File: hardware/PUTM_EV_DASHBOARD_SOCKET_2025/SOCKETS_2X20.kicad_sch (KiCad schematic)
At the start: 10 parts, among them J1pin200000 Conn_02x20_Top_Bottom_Mountin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, J2SO2 Conn_02x20_Top_Bottom_Mountin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

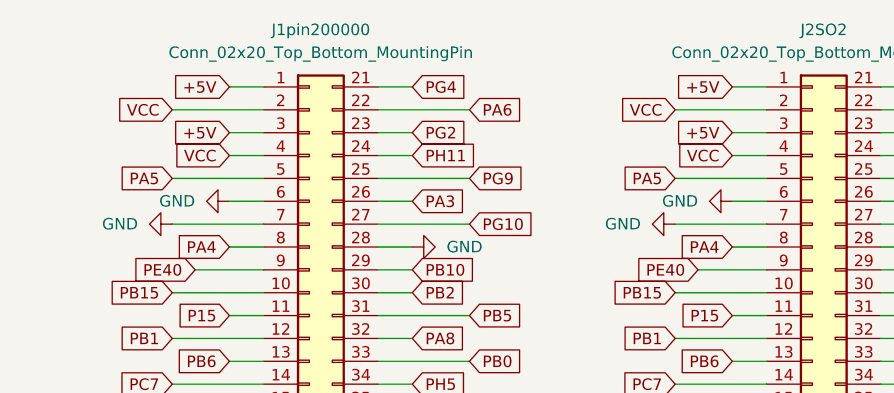
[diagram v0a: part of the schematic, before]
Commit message: gotowe
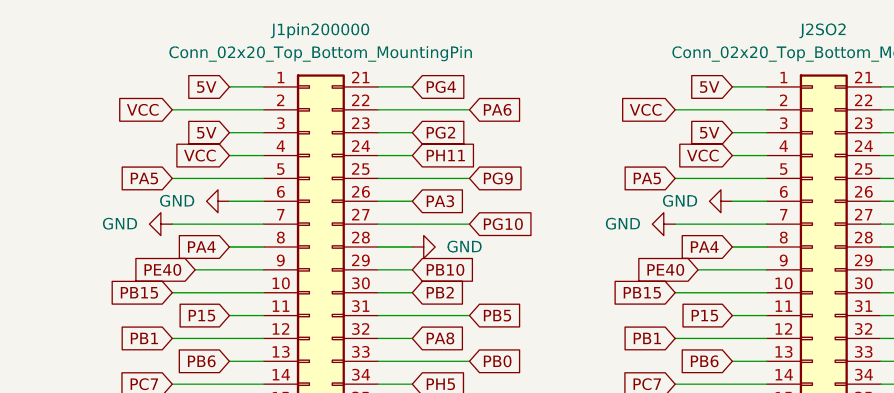
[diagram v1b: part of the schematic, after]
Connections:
- net +5V renamed 5V
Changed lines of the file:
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@@
 		)
 	)
-	(global_label "+5V"
+	(global_label "5V"
 		(shape input)
 		(at 168.91 66.04 180)
@@
 		)
 		(property "Intersheetrefs" "${INTERSHEET_REFS}"
-			(at 162.0543 66.04 0)
+			(at 163.6267 66.04 0)
 			(effects
 				(font
@@
 		)
 	)
-	(global_label "+5V"
+	(global_label "5V"
 		(shape input)
 		(at 113.03 66.04 180)
@@
 		)
 		(property "Intersheetrefs" "${INTERSHEET_REFS}"
-			(at 106.1743 66.04 0)
+			(at 107.7467 66.04 0)
 			(effects
 				(font
@@
 		)
 	)
-	(global_label "+5V"
+	(global_label "5V"
 		(shape input)
 		(at 168.91 60.96 180)
@@
 		)
 		(property "Intersheetrefs" "${INTERSHEET_REFS}"
-			(at 162.0543 60.96 0)
+			(at 163.6267 60.96 0)
 			(effects
 				(font
@@
 		)
 	)
-	(global_label "+5V"
+	(global_label "5V"
 		(shape input)
 		(at 113.03 60.96 180)
@@
 		)
 		(property "Intersheetrefs" "${INTERSHEET_REFS}"
-			(at 106.1743 60.96 0)
-			(effects
-				(font
+			(at 107.7467 60.96 0)
+			(effects
+				(font

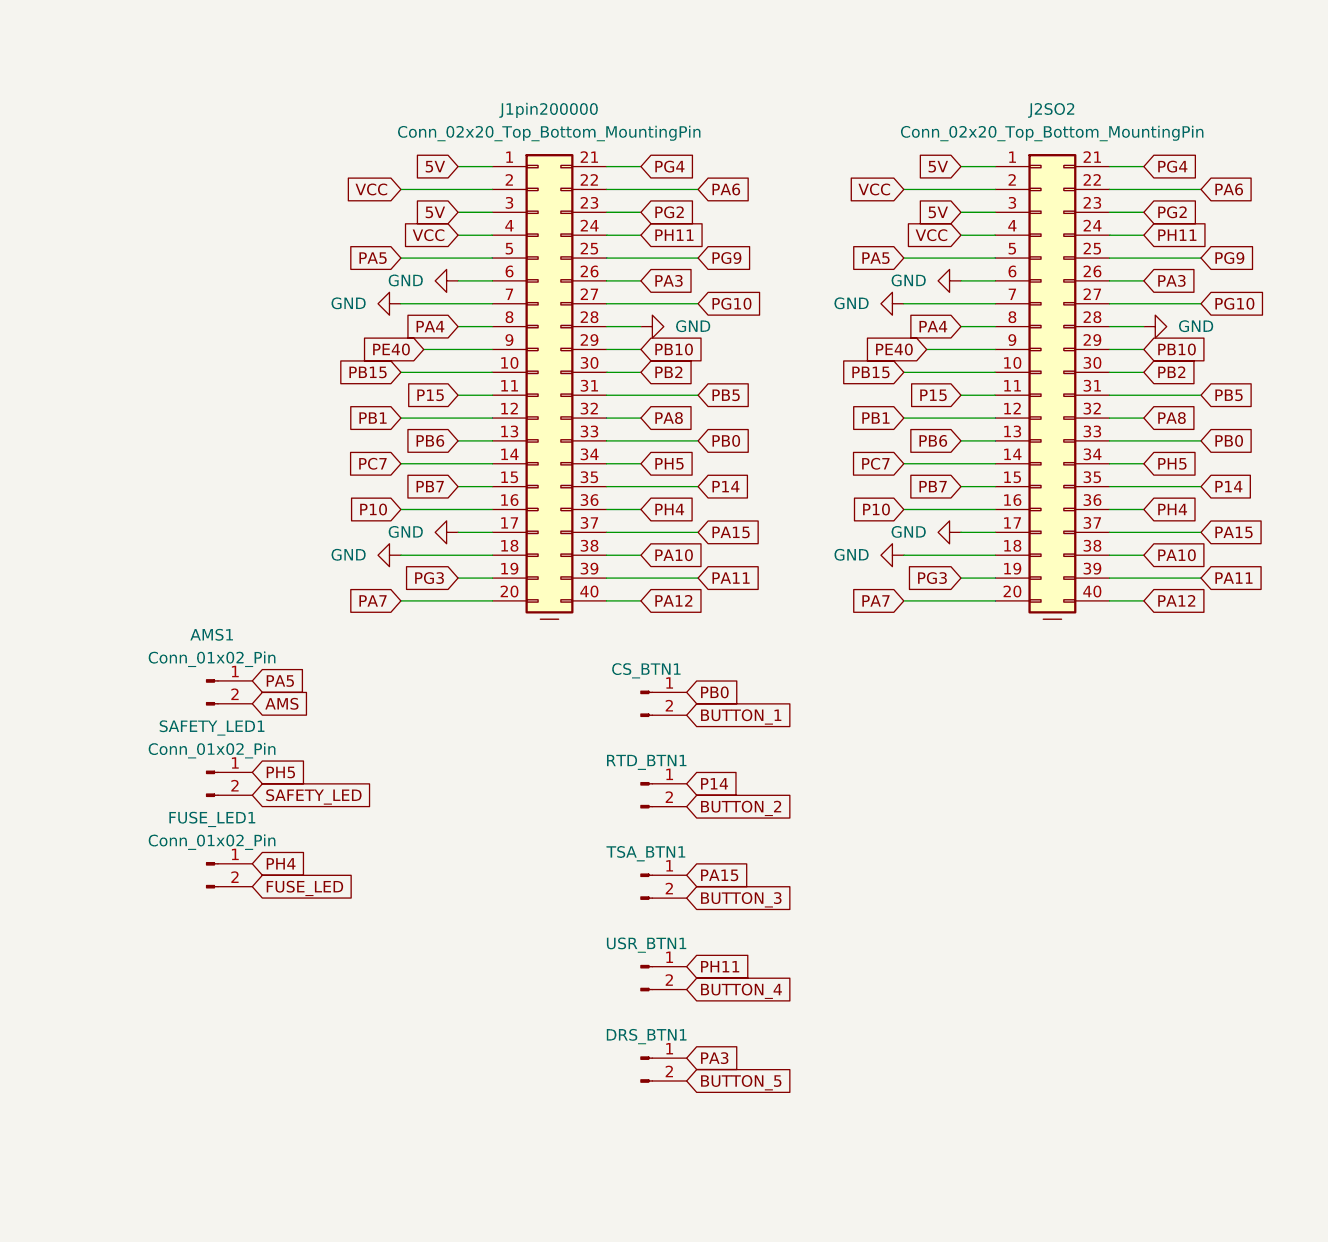
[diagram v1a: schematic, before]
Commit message: jest jako tako
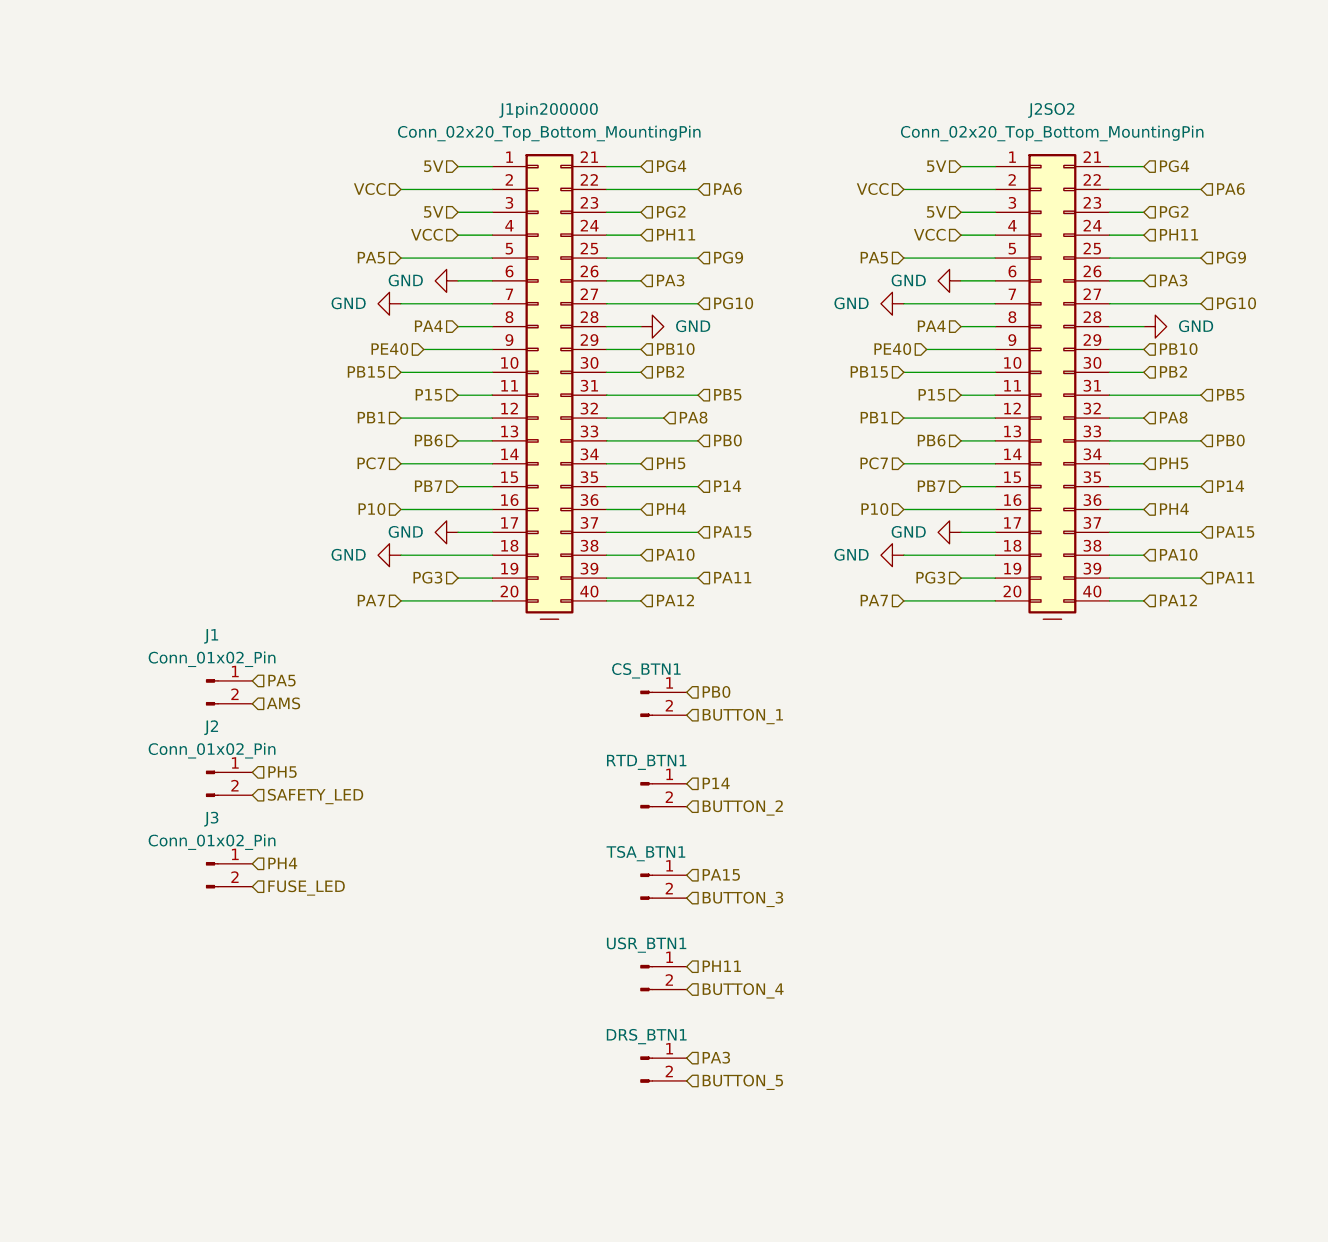
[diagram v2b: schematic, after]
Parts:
- renumbered AMS1 to J1, SAFETY_LED1 to J2, FUSE_LED1 to J3

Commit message: g3
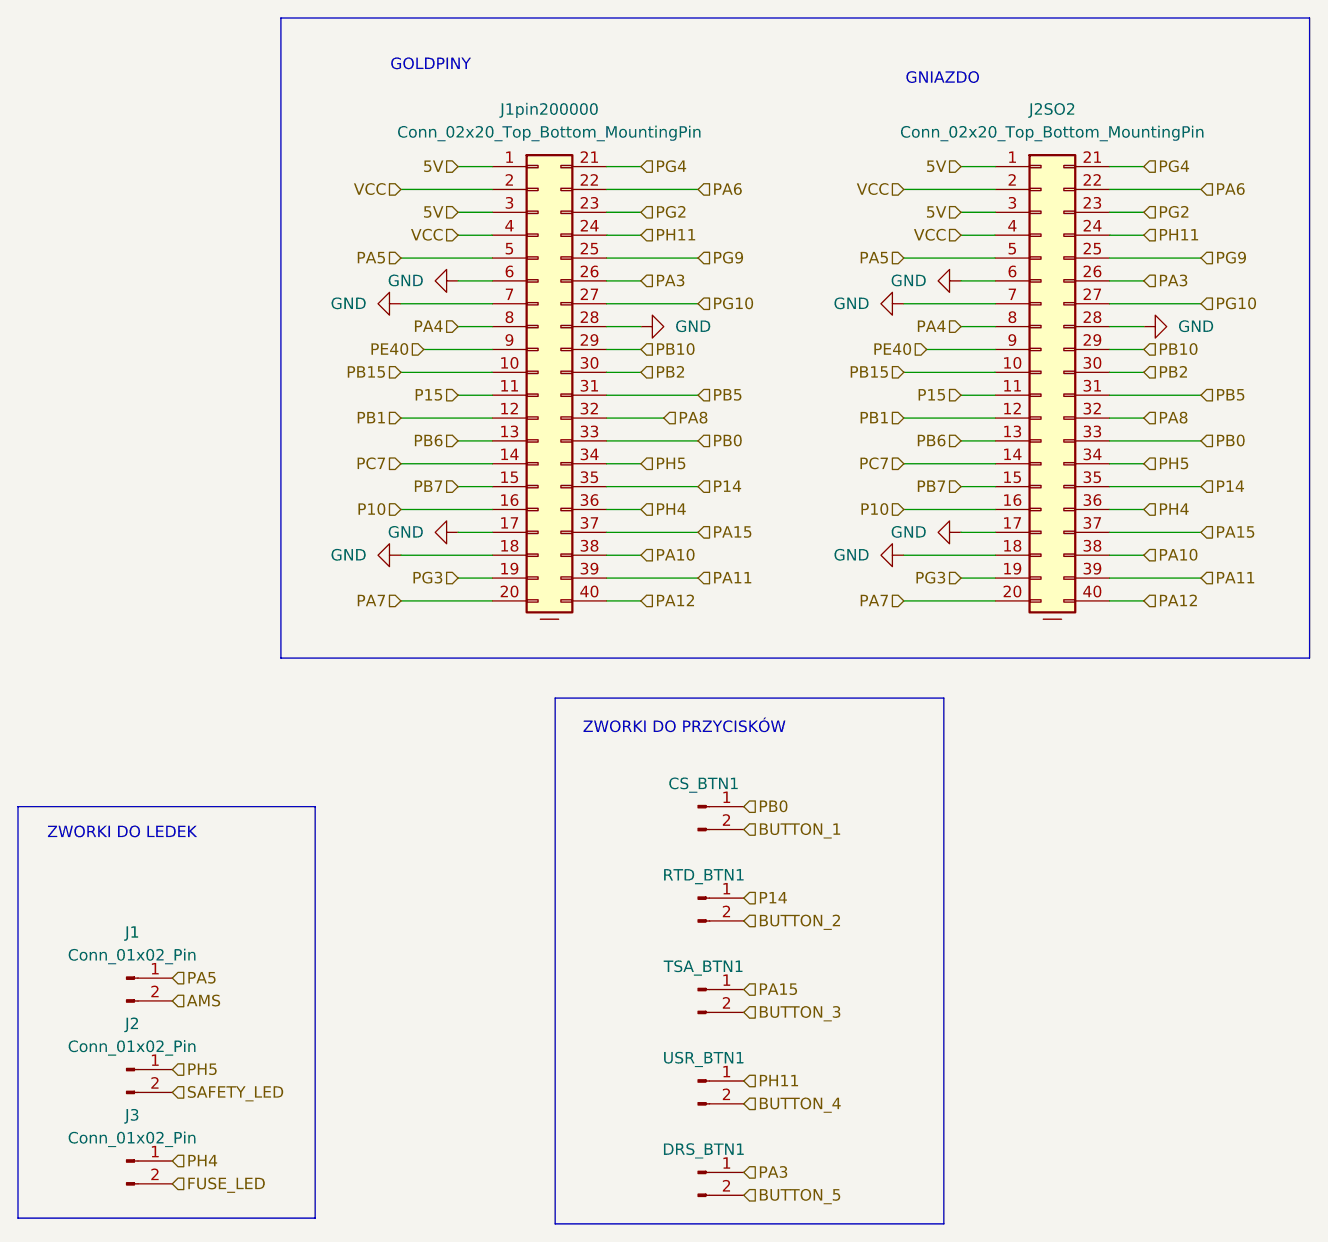
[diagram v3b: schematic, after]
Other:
- note added: "GNIAZDO"
- note added: "GOLDPINY"
- note added: "ZWORKI DO LEDEK"
- note added: "ZWORKI DO PRZYCISKÓW"
- moved on the sheet: CS_BTN1, DRS_BTN1, J1, J2, J3, RTD_BTN1, TSA_BTN1, USR_BTN1

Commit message: fixed button logic, holes for inserts, distance from mounting holes to P4 socket, changed jumpers, TVS diode and footprint for laboratory socket 4m
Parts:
- CS_BTN1, DRS_BTN1, J1, J2, J3, RTD_BTN1, TSA_BTN1, USR_BTN1: footprint Connector_PinHeader_1.27mm:PinHeader_1x02_P1.27mm_Vertical -> Connector_PinHeader_2.54mm:PinHeader_1x02_P2.54mm_Vertical
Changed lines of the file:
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@@
 			)
 		)
-		(property "Footprint" "Connector_PinHeader_1.27mm:PinHeader_1x02_P1.27mm_Vertical"
+		(property "Footprint" "Connector_PinHeader_2.54mm:PinHeader_1x02_P2.54mm_Vertical"
 			(at 76.2 161.29 0)
 			(effects
@@
 			)
 		)
-		(property "Footprint" "Connector_PinHeader_1.27mm:PinHeader_1x02_P1.27mm_Vertical"
+		(property "Footprint" "Connector_PinHeader_2.54mm:PinHeader_1x02_P2.54mm_Vertical"
 			(at 139.7 132.08 0)
 			(effects
@@
 			)
 		)
-		(property "Footprint" "Connector_PinHeader_1.27mm:PinHeader_1x02_P1.27mm_Vertical"
+		(property "Footprint" "Connector_PinHeader_2.54mm:PinHeader_1x02_P2.54mm_Vertical"
 			(at 139.7 162.56 0)
 			(effects
@@
 			)
 		)
-		(property "Footprint" "Connector_PinHeader_1.27mm:PinHeader_1x02_P1.27mm_Vertical"
+		(property "Footprint" "Connector_PinHeader_2.54mm:PinHeader_1x02_P2.54mm_Vertical"
 			(at 76.2 171.45 0)
 			(effects
@@
 			)
 		)
-		(property "Footprint" "Connector_PinHeader_1.27mm:PinHeader_1x02_P1.27mm_Vertical"
+		(property "Footprint" "Connector_PinHeader_2.54mm:PinHeader_1x02_P2.54mm_Vertical"
 			(at 76.2 151.13 0)
 			(effects
@@
 			)
 		)
-		(property "Footprint" "Connector_PinHeader_1.27mm:PinHeader_1x02_P1.27mm_Vertical"
+		(property "Footprint" "Connector_PinHeader_2.54mm:PinHeader_1x02_P2.54mm_Vertical"
 			(at 139.7 142.24 0)
 			(effects
@@
 			)
 		)
-		(property "Footprint" "Connector_PinHeader_1.27mm:PinHeader_1x02_P1.27mm_Vertical"
+		(property "Footprint" "Connector_PinHeader_2.54mm:PinHeader_1x02_P2.54mm_Vertical"
 			(at 139.7 172.72 0)
 			(effects
@@
 			)
 		)
-		(property "Footprint" "Connector_PinHeader_1.27mm:PinHeader_1x02_P1.27mm_Vertical"
+		(property "Footprint" "Connector_PinHeader_2.54mm:PinHeader_1x02_P2.54mm_Vertical"
 			(at 139.7 152.4 0)
 			(effects
